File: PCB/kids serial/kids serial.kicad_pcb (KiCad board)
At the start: 2 copper layers, 76.2 x 43.2 mm, 15 parts, among them J1 n8 Bus Connector, U1 SC28L92_PLC44, U2 FT230XS, X1 3.6864Mhz

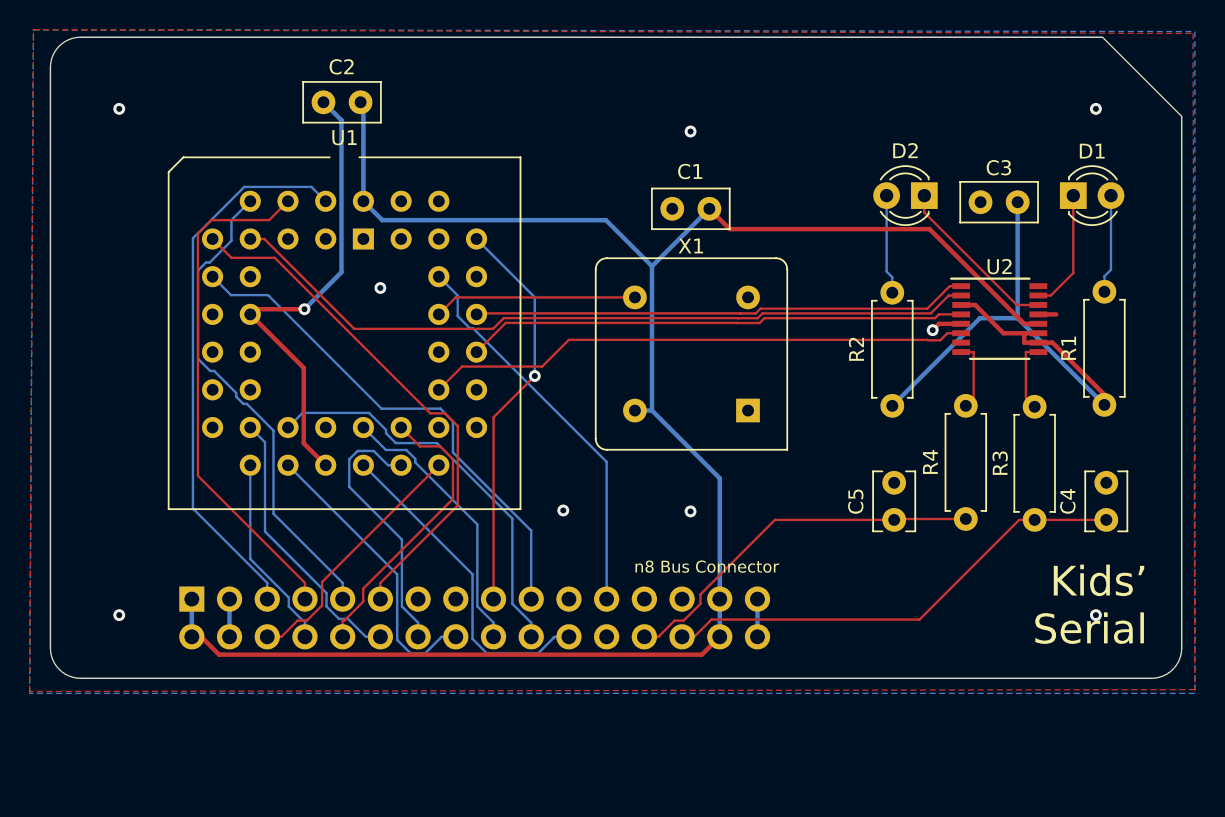
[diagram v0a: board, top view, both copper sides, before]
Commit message: v2 changes
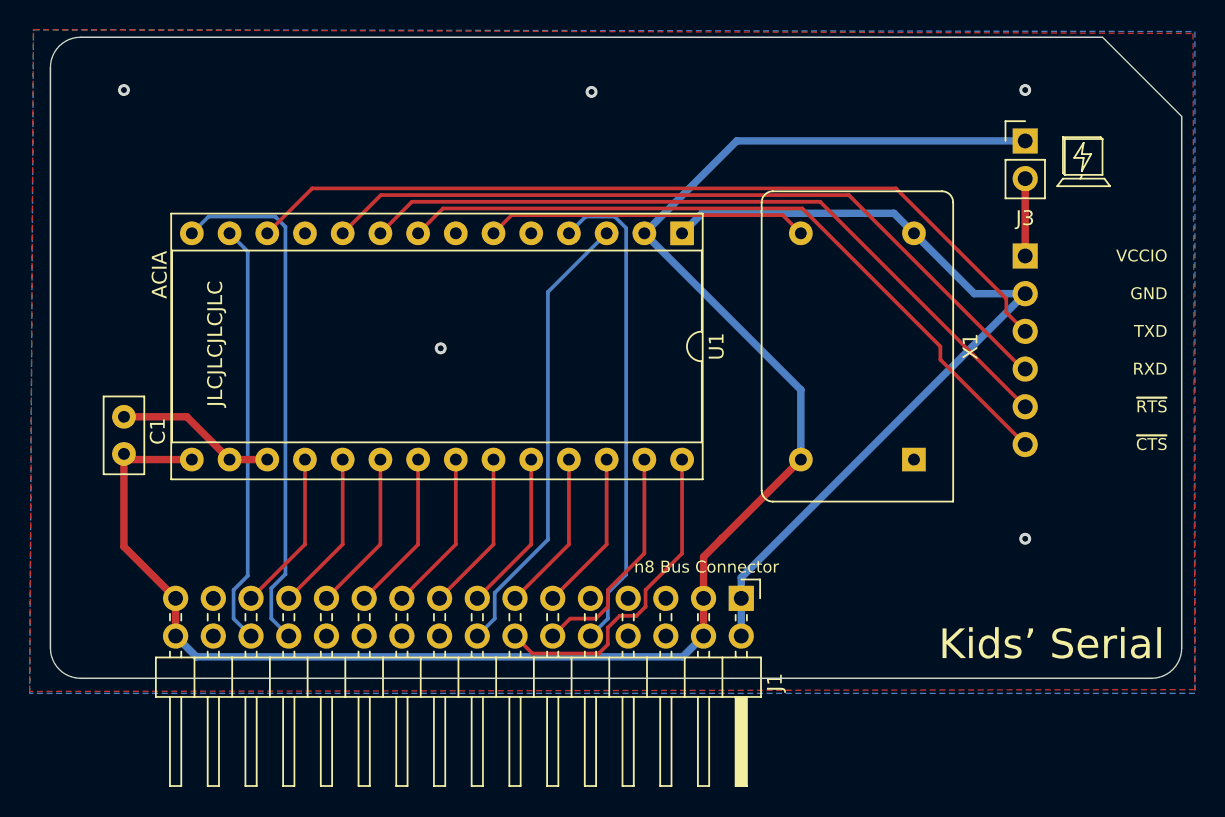
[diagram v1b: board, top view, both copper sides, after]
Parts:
- removed C2, C3: 100nF, Capacitor_THT:C_Disc_D5.0mm_W2.5mm_P2.50mm
- removed C4, C5: 47pF, Capacitor_THT:C_Disc_D3.8mm_W2.6mm_P2.50mm
- removed D1: TX, LED_THT:LED_D3.0mm
- removed D2: RX, LED_THT:LED_D3.0mm
- removed R1, R2: 330, Resistor_THT:R_Axial_DIN0207_L6.3mm_D2.5mm_P7.62mm_Horizontal
- removed R3, R4: 27, Resistor_THT:R_Axial_DIN0207_L6.3mm_D2.5mm_P7.62mm_Horizontal
- removed U2: FT230XS, Package_SO:SSOP-16_3.9x4.9mm_P0.635mm
- added J2: UARTConnector, Connector_PinSocket_2.54mm:PinSocket_1x06_P2.54mm_Horizontal, B.Cu at (166.2, 89.5)
- added J3: PowerViaUSB, Connector_PinHeader_2.54mm:PinHeader_1x02_P2.54mm_Vertical, F.Cu at (166.2, 81.8)
- C1: value 100nF -> 100nf
- J1: moved to F.Cu
- U1: value SC28L92_PLC44 -> 6551; footprint Package_LCC:PLCC-44_THT-Socket -> Package_DIP:DIP-28_W15.24mm_Socket
- X1: value 3.6864Mhz -> CXO_DIP14; footprint Oscillator:Oscillator_DIP-8 -> Oscillator:Oscillator_DIP-14
- moved C1 42.7 mm to (105.5, 102.9), turned to 90 degrees
- moved J1 37.0 mm to (147.1, 112.6)
- moved U1 21.5 mm to (143.1, 88.0), turned to 270 degrees
- moved X1 11.7 mm to (158.8, 103.3)
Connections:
- J1 pad 1: +5V -> GND
- J1 pad 10: /D2 -> ~RES
- J1 pad 11: /A3 -> ~IRQ
- J1 pad 12: /D3 -> CLK
- J1 pad 13: /A4 -> /D7
- J1 pad 14: /D4 -> R~W
- J1 pad 15: /A5 -> /D6
- J1 pad 16: /D5 -> ~CS
- J1 pad 17: ~CS -> /D5
- J1 pad 18: /D6 -> /A5
- J1 pad 19: R~W -> /D4
- J1 pad 2: +5V -> GND
- J1 pad 20: /D7 -> /A4
- J1 pad 21: CLK -> /D3
- J1 pad 22: ~IRQ -> /A3
- J1 pad 23: ~RES -> /D2
- J1 pad 24: Net-(J1-Pad24) -> /A2
- J1 pad 25: Net-(J1-Pad25) -> /D1
- J1 pad 26: USB_D+ -> /A1
- J1 pad 27: Net-(J1-Pad27) -> /D0
- J1 pad 28: USB_D- -> /A0
- J1 pad 29: +5V -> GND
- J1 pad 3: GND -> +5V
- J1 pad 30: +5V -> GND
- J1 pad 31: GND -> +5V
- J1 pad 32: GND -> +5V
- J1 pad 4: GND -> +5V
- J1 pad 5: /A0 -> Net-(J1-Pad5)
- J1 pad 6: /D0 -> Net-(J1-Pad6)
- J1 pad 7: /A1 -> Net-(J1-Pad7)
- J1 pad 8: /D1 -> Net-(J1-Pad8)
- J1 pad 9: /A2 -> Net-(J1-Pad9)
- U1 pad 1: Net-(U1-Pad1) -> GND
- U1 pad 10: Net-(U1-Pad10) -> RXD_IO
- U1 pad 12: GND -> TXD_IO
- U1 pad 13: Net-(U1-Pad13) -> /A0
- U1 pad 14: Net-(U1-Pad14) -> /A1
- U1 pad 15: Net-(U1-Pad15) -> +5V
- U1 pad 16: Net-(U1-Pad16) -> GND
- U1 pad 17: Net-(U1-Pad17) -> GND
- U1 pad 18: /D1 -> /D0
- U1 pad 19: /D3 -> /D1
- U1 pad 2: /A0 -> +5V
- U1 pad 20: /D5 -> /D2
- U1 pad 21: /D7 -> /D3
- U1 pad 22: GND -> /D4
- U1 pad 23: Net-(U1-Pad23) -> /D5
- U1 pad 24: ~IRQ -> /D6
- U1 pad 25: /D6 -> /D7
- U1 pad 26: /D4 -> ~IRQ
- U1 pad 27: /D2 -> CLK
- U1 pad 28: /D0 -> R~W
- U1 pad 3: Net-(U1-Pad3) -> ~CS
- U1 pad 4: /A1 -> ~RES
- U1 pad 6: /A2 -> XTAL_CLK
- U1 pad 7: /A3 -> Net-(U1-Pad7)
- U1 pad 8: ~CTS -> ~CTS_IO
- U1 pad 9: R~W -> ~RTS_IO
- X1 pad 8: +5V -> XTAL_CLK
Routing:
- net TXD_IO: track 0.00 -> 56.8 mm
- net RXD_IO: track 0.00 -> 51.9 mm
- net ~CTS: track 51.3 -> 0.00 mm
- net ~RTS_IO: track 0.00 -> 50.0 mm
- net ~CTS_IO: track 0.00 -> 48.7 mm
- net +3V3: track 41.1 -> 0.00 mm
- net ~RTS: track 36.8 -> 0.00 mm
- net /A3: track 35.5 -> 0.00 mm
- net TxD: track 33.7 -> 0.00 mm
- net RxD: track 33.4 -> 0.00 mm
- net /A2: track 32.7 -> 0.00 mm
- net USB_D-: track 31.8 -> 0.00 mm
- net GND: track 40.0 -> 67.7 mm, vias 10 -> 5
- net USB_D+: track 25.3 -> 0.00 mm
- net /D7: track 27.1 -> 10.9 mm
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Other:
- net class Default: clearance 0.16 -> 0.2; trace_width 0.16 -> 0.25
- net class Power: clearance 0.2 -> 0.3; trace_width 0.3 -> 0.5
- rule trace_clearance: 0.16 -> 0.2
- rule trace_min: 0.154 -> 0.2
- board text added: "ACIA"
- board text added: "GND"
- board text added: "JLCJLCJLCJLC"
- board text added: "RXD"
- board text added: "TXD"
- board text added: "VCCIO"
- board text added: "~CTS"
- board text added: "~RTS"
